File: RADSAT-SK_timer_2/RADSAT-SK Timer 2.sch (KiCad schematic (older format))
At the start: 70 parts, among them J201 Conn_01x07, J202 Conn_01x05_Female, J203 Conn_01x03, J204 Conn_01x02, J205 Conn_01x02, J206 Conn_01x02, J207 Conn_02x26_Odd_Even, J208 Conn_02x26_Odd_Even, Q204 IRLML2060, Q205 IRLML2060, Q206 IRLML2060, SW201 SW_Push, SW202 SW_Push, SW203 SW_Push, SW204 SW_Push, SW205 SW_Push, SW206 SW_Push, U101 LT1521, U102 Galaxia_Timer, U202 TPS3700DDCR, U230 CPC1114N, U240 CPC1114N, U250 CPC1114N, U260 CPC1114N

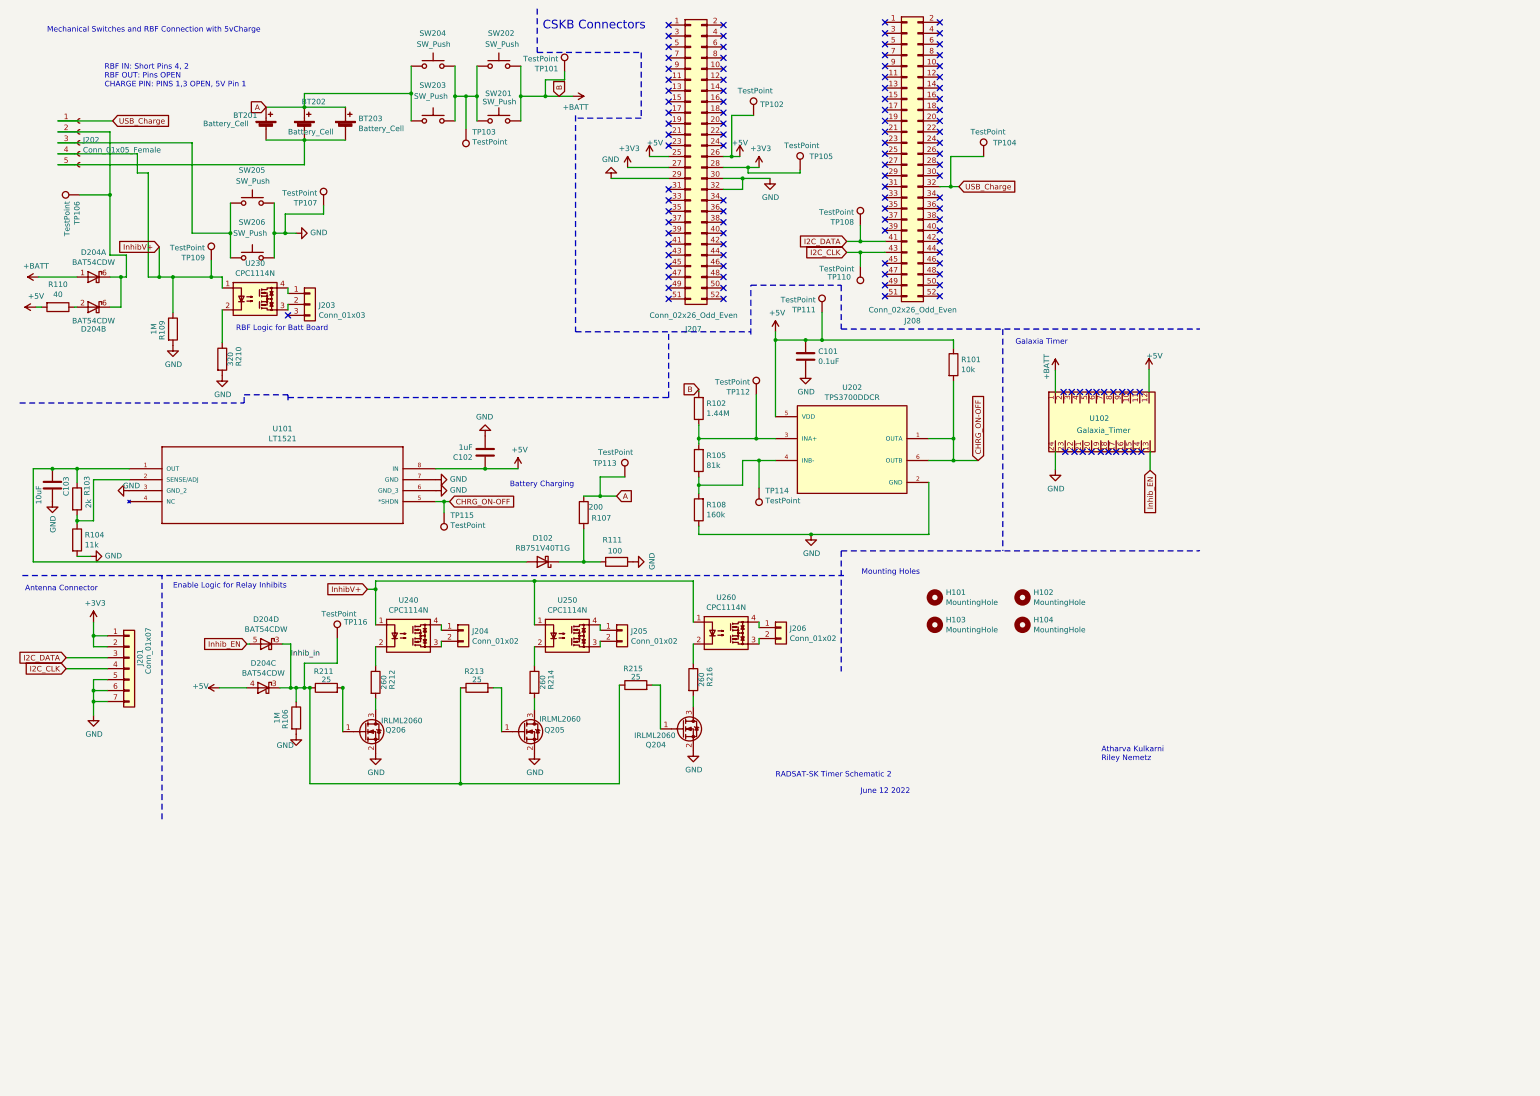
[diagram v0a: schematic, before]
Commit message: 555 push for production
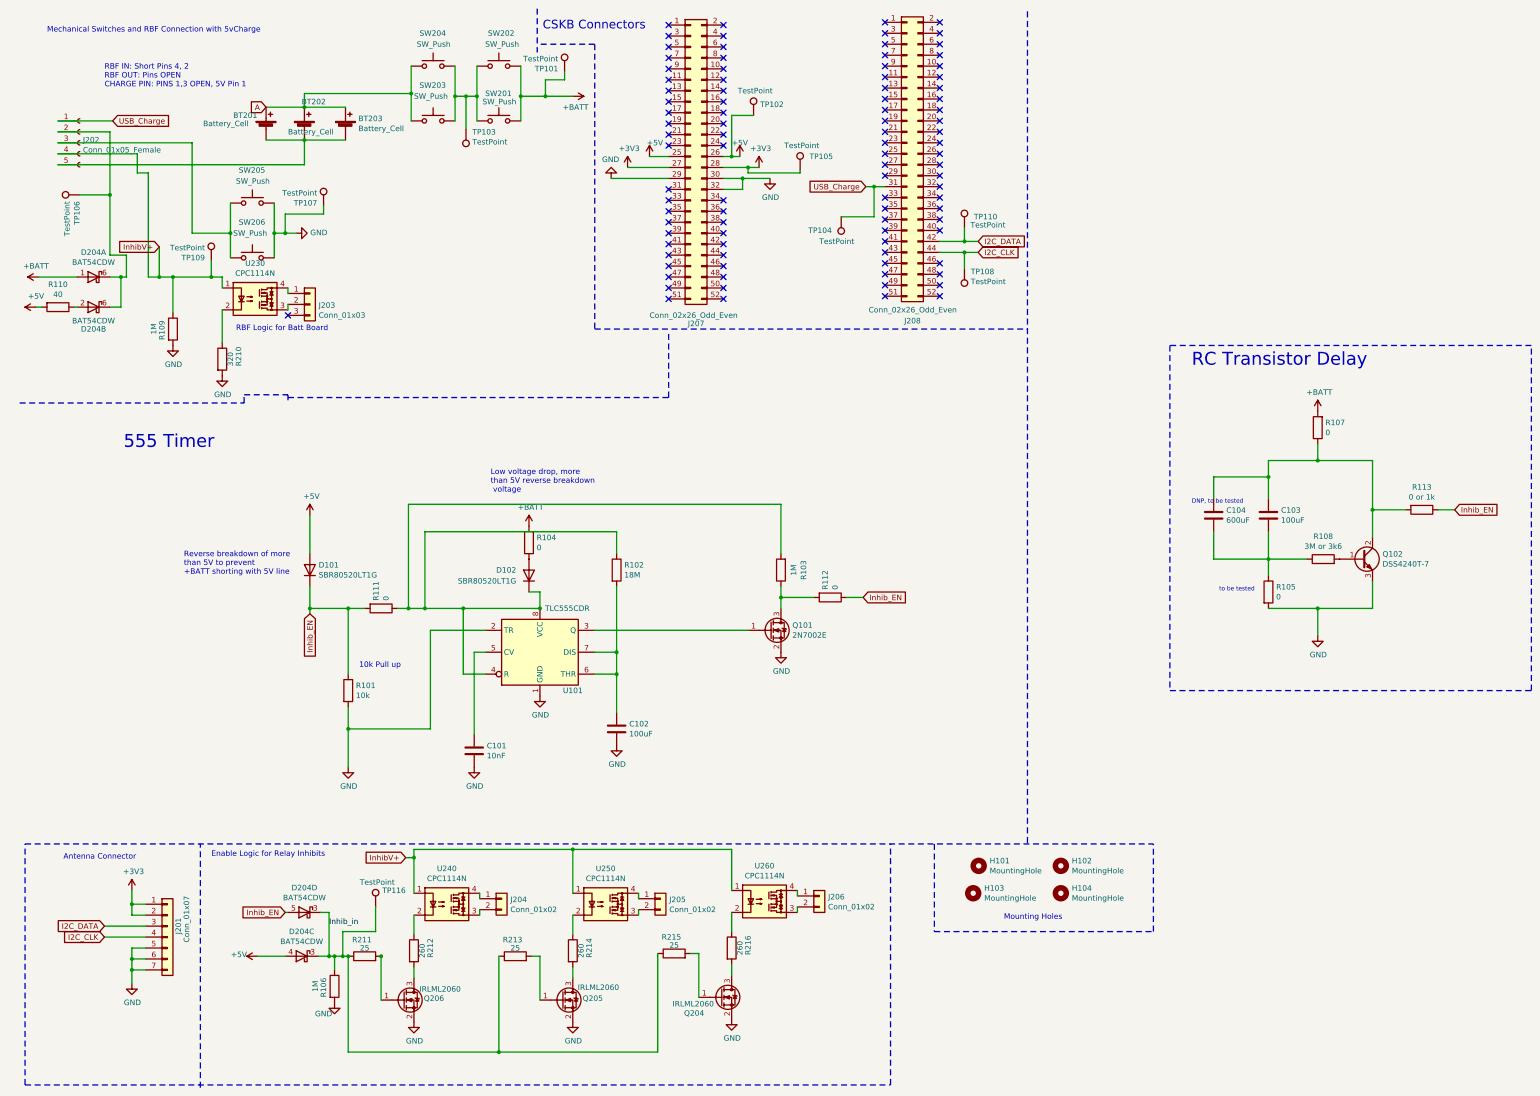
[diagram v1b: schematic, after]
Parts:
- removed D102: RB751V40T1G, Diode_SMD:D_SOD-323, symbol Device:D_Schottky
- removed TP111, TP112, TP113, TP114, TP115: TestPoint, S2761-46R:HARWIN_S2761-46R, symbol Connector:TestPoint
- removed U101: LT1521, LT1521IS8-5TR:SO-8_S, symbol LT1521IS8-5TR:LT1521IS8-5TR
- removed U102: Galaxia_Timer, Galaxia_Timer:Galaxia_Timer, symbol Galaxia_Timer:Galaxia_Timer
- removed U202: TPS3700DDCR, Package_TO_SOT_SMD:TSOT-23-6, symbol RADSAT-SK-Timer-rescue:TPS3700DDCR-TPS3700DDCR
- added C104: 600uF, Capacitor_SMD:C_1206_3216Metric, symbol Device:C
- added D101, D102: SBR80520LT1G, Diode_SMD:D_SOD-123, symbol Device:D
- added Q101: 2N7002E, Package_TO_SOT_SMD:SOT-23, symbol Transistor_FET:2N7002E
- added Q102: DSS4240T-7, Package_TO_SOT_SMD:SOT-23, symbol Device:Q_NPN_BCE
- added R112: 0, Resistor_SMD:R_1206_3216Metric_Pad1.30x1.75mm_HandSolder, symbol Device:R
- added R113: 0 or 1k, Resistor_SMD:R_1206_3216Metric_Pad1.30x1.75mm_HandSolder, symbol Device:R
- added U101: TLC555CDR, Package_SO:SOIC-8_3.9x4.9mm_P1.27mm, symbol Timer:TLC555xD
- C101: value 0.1uF -> 10nF; footprint Capacitor_SMD:C_0805_2012Metric -> Capacitor_SMD:C_1206_3216Metric
- C102: value 1uF -> 100uF; footprint Capacitor_SMD:C_0805_2012Metric -> Capacitor_SMD:C_1206_3216Metric
- C103: value 10uF -> 100uF; footprint Capacitor_SMD:C_0805_2012Metric -> Capacitor_SMD:C_1206_3216Metric
- R101: footprint Resistor_SMD:R_0805_2012Metric -> Resistor_SMD:R_1206_3216Metric_Pad1.30x1.75mm_HandSolder
- R102: value 1.44M -> 18M; footprint Resistor_SMD:R_0805_2012Metric -> Resistor_SMD:R_1206_3216Metric_Pad1.30x1.75mm_HandSolder
- R103: value 2k -> 1M; footprint Resistor_SMD:R_0805_2012Metric -> Resistor_SMD:R_1206_3216Metric_Pad1.30x1.75mm_HandSolder
- R104: value 11k -> 0; footprint Resistor_SMD:R_0805_2012Metric -> Resistor_SMD:R_1206_3216Metric_Pad1.30x1.75mm_HandSolder
- R105: value 81k -> 0; footprint Resistor_SMD:R_0805_2012Metric -> Resistor_SMD:R_1206_3216Metric_Pad1.30x1.75mm_HandSolder
- R107: value 200 -> 0; footprint Resistor_SMD:R_0805_2012Metric -> Resistor_SMD:R_1206_3216Metric_Pad1.30x1.75mm_HandSolder
- R108: value 160k -> 3M or 3k6; footprint Resistor_SMD:R_0805_2012Metric -> Resistor_SMD:R_1206_3216Metric_Pad1.30x1.75mm_HandSolder
- R111: value 100 -> 0; footprint Resistor_THT:R_Axial_DIN0309_L9.0mm_D3.2mm_P12.70mm_Horizontal -> Resistor_SMD:R_1206_3216Metric_Pad1.30x1.75mm_HandSolder
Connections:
- net CHRG_ON-OFF is gone; now on net GND: R101.2
- net +5V: now also D101.2 (A); no longer C101.1, C102.1, R101.1
- net +BATT: now also R104.2, R107.2; no longer R102.2
- net A: no longer R107.1
- net GND: now also R105.2, Q101.2 (S), Q102.3 (E), U101.1 (GND), U101.2 (TR); no longer C103.2, R104.2, R108.1, R111.1
- net I2C_CLK: now also J208.44 (Pin_44), TP108.1; no longer J208.43 (Pin_43), TP110.1
- net I2C_DATA: now also J208.42 (Pin_42), TP110.1; no longer J208.41 (Pin_41), TP108.1
- net Inhib_EN: now also R101.1, R111.2, D101.1 (K), R112.1, R113.1
- net USB_Charge: now also J208.31 (Pin_31); no longer J208.32 (Pin_32)
- net at R103.1: now also Q101.3 (D), R112.2; no longer C103.1
- net at R103.2: now also R102.1, R111.1, D102.1 (K), U101.4 (R), U101.8 (VCC); no longer R104.1
- net at R105.1: now also C103.2, R108.1, C104.2; no longer R108.2
- new net: Q101.1 (G), U101.3 (Q)
- new net: C101.1, U101.5 (CV)
- new net: C102.1, R102.2, U101.6 (THR), U101.7 (DIS)
- new net: D102.2 (A), R104.1
- new net: Q102.1 (B), R108.2
- new net: C103.1, C104.1, Q102.2 (C), R107.1, R113.2
- no-connect marks 115 -> 95
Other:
- note added: "10k Pull up\n"
- note added: "555 Timer"
- note added: "DNP, to be tested"
- note added: "Low voltage drop, more \nthan 5V reverse breakdown\n voltage\n"
- note added: "RC Transistor Delay \n"
- note added: "Reverse breakdown of more \nthan 5V to prevent \n+BATT shorting with 5V line\n"
- note added: "to be tested\n"
- note removed: "Atharva Kulkarni\nRiley Nemetz\n"
- note removed: "Battery Charging\n"
- note removed: "Galaxia Timer\n"
- note removed: "June 12 2022"
- note removed: "RADSAT-SK Timer Schematic 2"
- moved on the sheet: D204C, D204D, H101, H102, H103, H104, J201, J204, J205, J206, Q204, Q205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
